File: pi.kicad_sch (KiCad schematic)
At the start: 3 parts, among them J33 2540-5

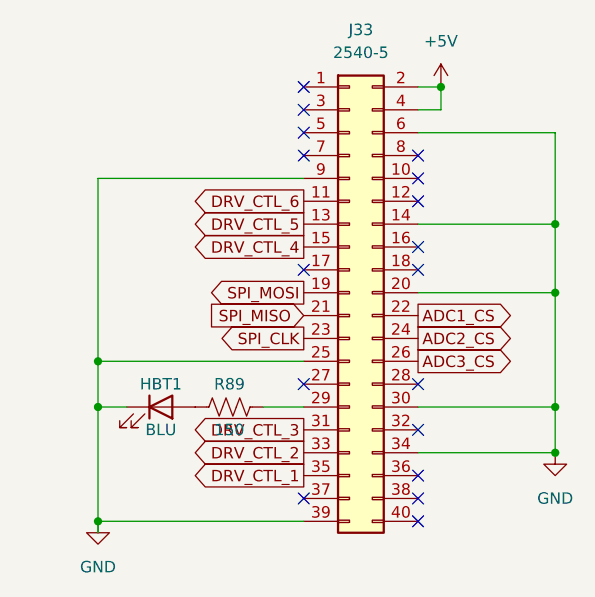
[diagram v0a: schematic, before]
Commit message: done schematiccing after design review
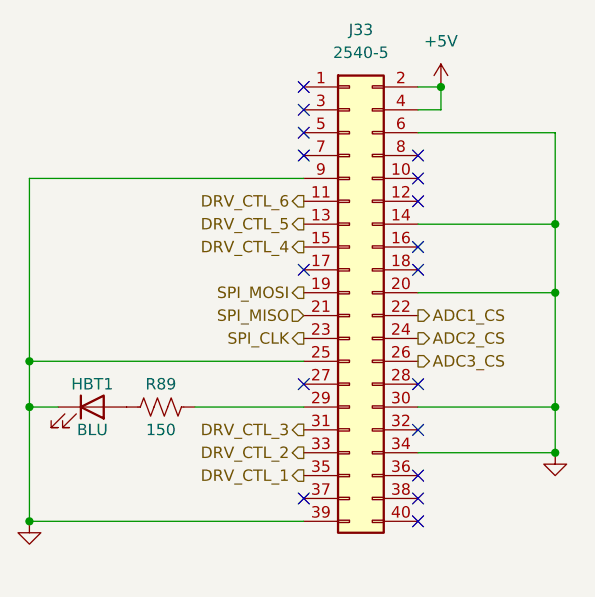
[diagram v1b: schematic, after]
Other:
- moved on the sheet: HBT1, R89

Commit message: final rev for jlc
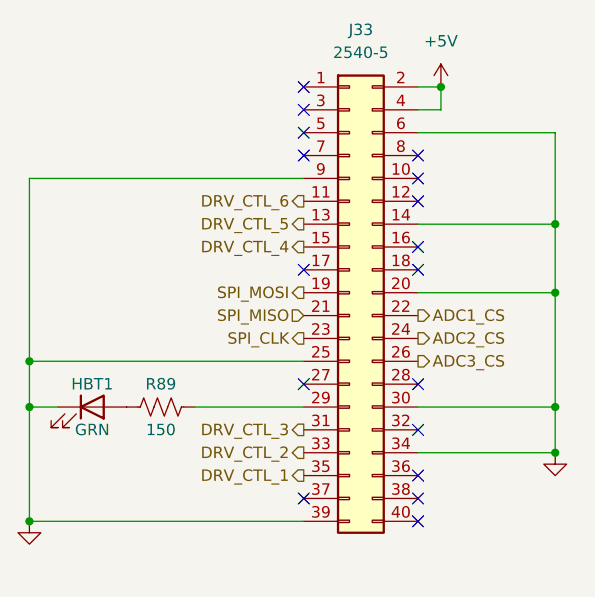
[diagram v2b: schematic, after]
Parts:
- HBT1: value BLU -> GRN
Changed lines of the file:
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@@
     (in_bom yes) (on_board yes)
     (property "Reference" "HBT1" (id 0) (at 75.565 95.25 0))
-    (property "Value" "BLU" (id 1) (at 75.565 100.33 0))
+    (property "Value" "GRN" (id 1) (at 75.565 100.33 0))
     (property "Footprint" "LED_SMD:LED_1206_3216Metric" (id 2) (at 75.565 97.79 0)
       (effects (font (size 1.27 1.27)) hide)

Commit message: my body is a machine that takes in peanut m&ms and puts out rocket engine controllers
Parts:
- HBT1: LCSC (none) -> C499462
- R89: LCSC (none) -> C17917
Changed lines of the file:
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@@
+      (effects (font (size 1.27 1.27)) hide)
+    )
+    (property "LCSC" "C17917" (id 4) (at 83.185 97.79 0)
       (effects (font (size 1.27 1.27)) hide)
     )
@@
       (effects (font (size 1.27 1.27)) hide)
     )
+    (property "LCSC" "C499462" (id 4) (at 75.565 97.79 0)
+      (effects (font (size 1.27 1.27)) hide)
+    )
